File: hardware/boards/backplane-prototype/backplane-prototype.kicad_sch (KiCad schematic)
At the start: 32 parts, among them J1 DC_IN, J2 SLOT_1, J3 SLOT_2, J4 SLOT_3, J5 SLOT_4, J6 SLOT_5, J7 SLOT_6, J8 i2c_busses

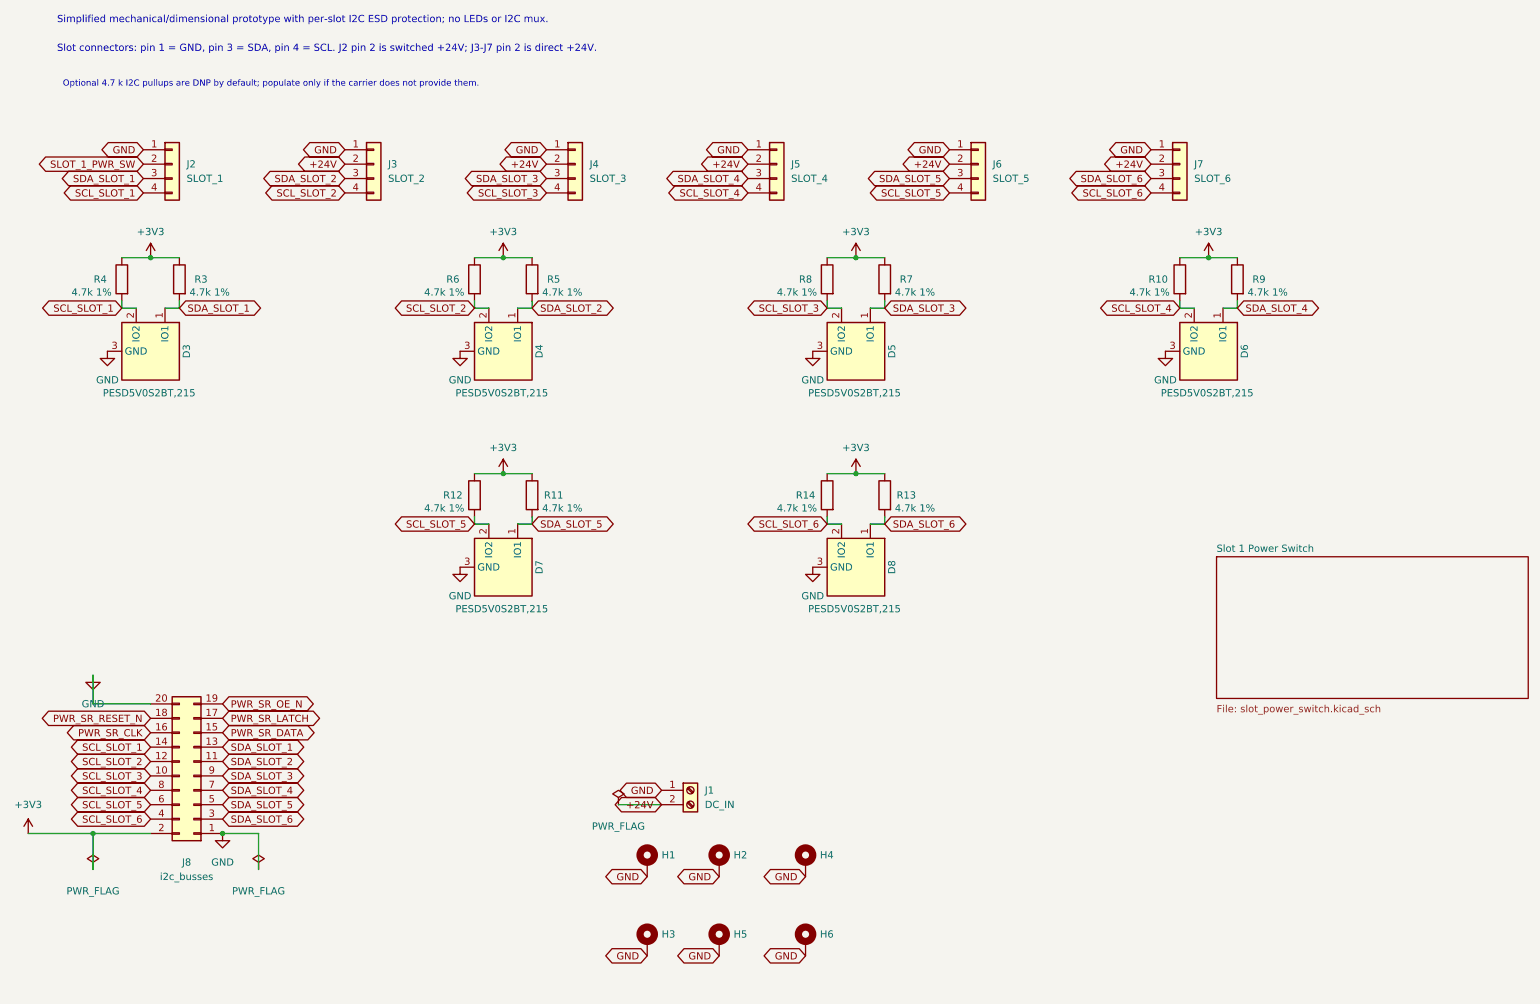
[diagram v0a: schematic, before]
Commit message: chore: checkpoint current board layout
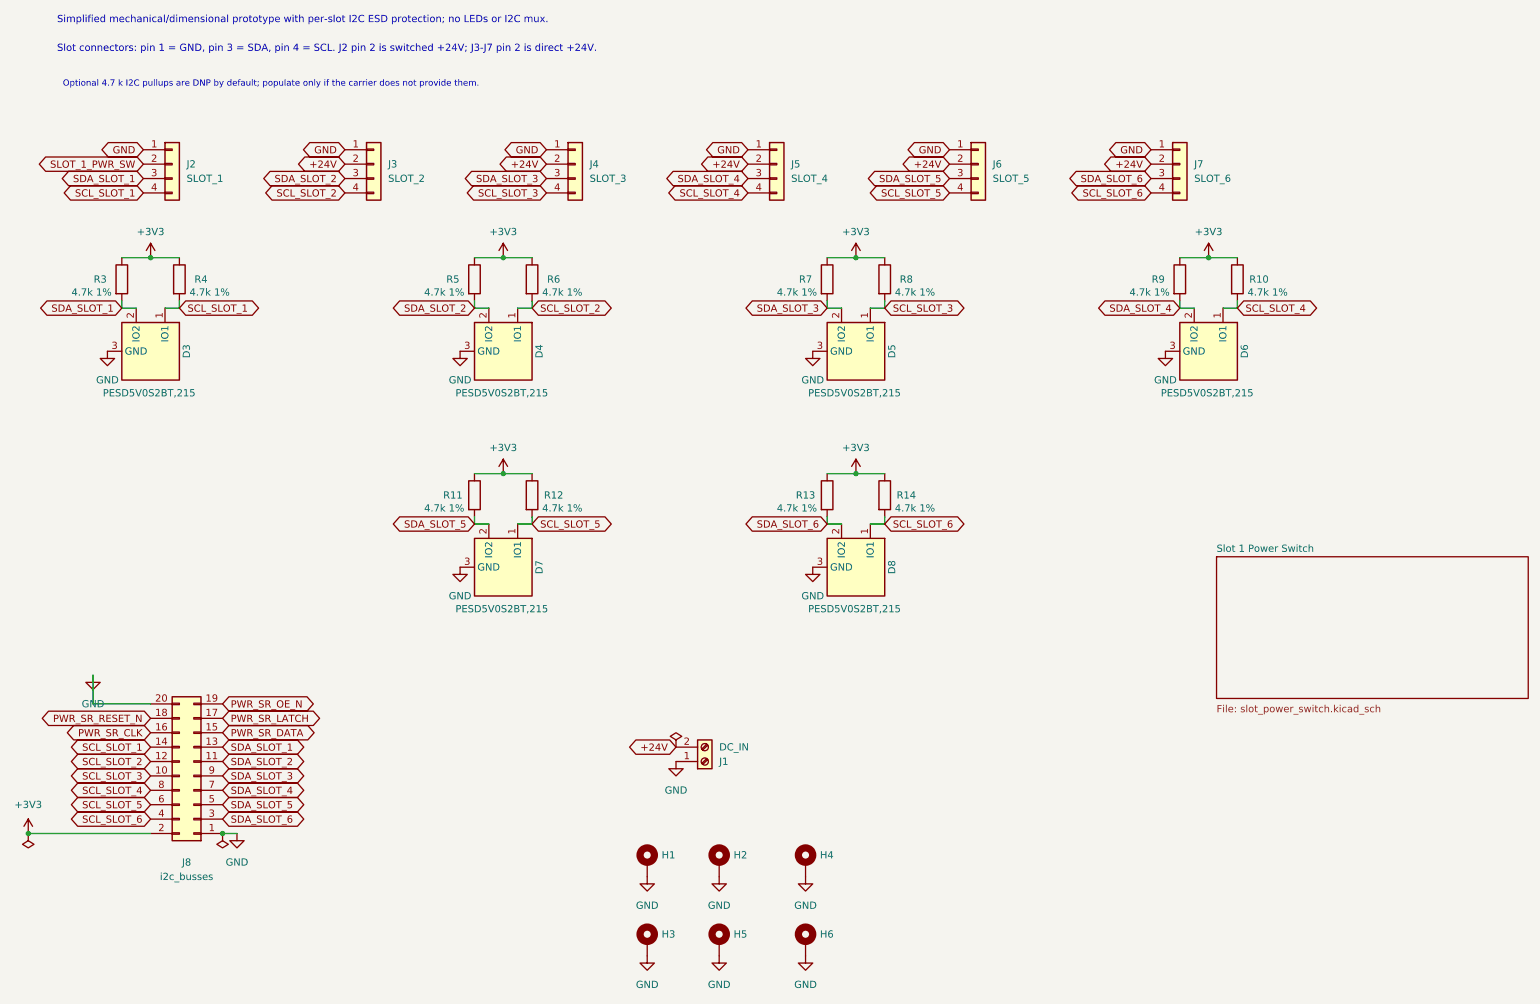
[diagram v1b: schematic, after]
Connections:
- net SCL_SLOT_1: now also D3.1 (IO1); no longer D3.2 (IO2)
- net SCL_SLOT_2: now also D4.1 (IO1); no longer D4.2 (IO2)
- net SCL_SLOT_3: now also D5.1 (IO1); no longer D5.2 (IO2)
- net SCL_SLOT_4: now also D6.1 (IO1); no longer D6.2 (IO2)
- net SCL_SLOT_5: now also D7.1 (IO1); no longer D7.2 (IO2)
- net SCL_SLOT_6: now also D8.1 (IO1); no longer D8.2 (IO2)
- net SDA_SLOT_1: now also D3.2 (IO2); no longer D3.1 (IO1)
- net SDA_SLOT_2: now also D4.2 (IO2); no longer D4.1 (IO1)
- net SDA_SLOT_3: now also D5.2 (IO2); no longer D5.1 (IO1)
- net SDA_SLOT_4: now also D6.2 (IO2); no longer D6.1 (IO1)
- net SDA_SLOT_5: now also D7.2 (IO2); no longer D7.1 (IO1)
- net SDA_SLOT_6: now also D8.2 (IO2); no longer D8.1 (IO1)
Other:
- title: Simplified XT30 Backplane Prototype -> Backplane Prototype
- moved on the sheet: J1, R10, R11, R12, R13, R14, R3, R4, R5, R6, R7, R8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
